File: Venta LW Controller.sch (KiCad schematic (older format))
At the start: 21 parts, among them J1 Conn_01x04, J2 Conn_02x05_Odd_Even, Q1 BSS138, Q2 BSS138, SW1 RST, SW2 FLASH, U1 LM2674N-3.3, U2 ESP32-WROOM-32

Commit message: updated parts
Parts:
- C1: footprint Capacitor_Tantalum_SMD:CP_EIA-3216-18_Kemet-A -> Capacitor_Tantalum_SMD:CP_EIA-7343-31_Kemet-D; Supplier Part TPSA226K010R0900 -> T491D226K035AT
- C4: Supplier Part CL03B103KP3NNNC -> CL21B103KBANNNC
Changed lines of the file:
@@
 F 0 "C1" H 1838 1696 50  0000 L CNN
 F 1 "22uF" H 1838 1605 50  0000 L CNN
-F 2 "Capacitor_Tantalum_SMD:CP_EIA-3216-18_Kemet-A" H 1750 1650 50  0001 C CNN
+F 2 "Capacitor_Tantalum_SMD:CP_EIA-7343-31_Kemet-D" H 1750 1650 50  0001 C CNN
 F 3 "~" H 1750 1650 50  0001 C CNN
 F 4 "TME" H 1750 1650 50  0001 C CNN "Supplier"
-F 5 "TPSA226K010R0900" H 1750 1650 50  0001 C CNN "Supplier Part"
+F 5 "T491D226K035AT" H 1750 1650 50  0001 C CNN "Supplier Part"
 	1    1750 1650
 	1    0    0    -1
@@
 F 3 "~" H 2600 2550 50  0001 C CNN
 F 4 "TME" H 2600 2550 50  0001 C CNN "Supplier"
-F 5 "CL03B103KP3NNNC" H 2600 2550 50  0001 C CNN "Supplier Part"
+F 5 "CL21B103KBANNNC" H 2600 2550 50  0001 C CNN "Supplier Part"
 	1    2600 2550
 	1    0    0    -1

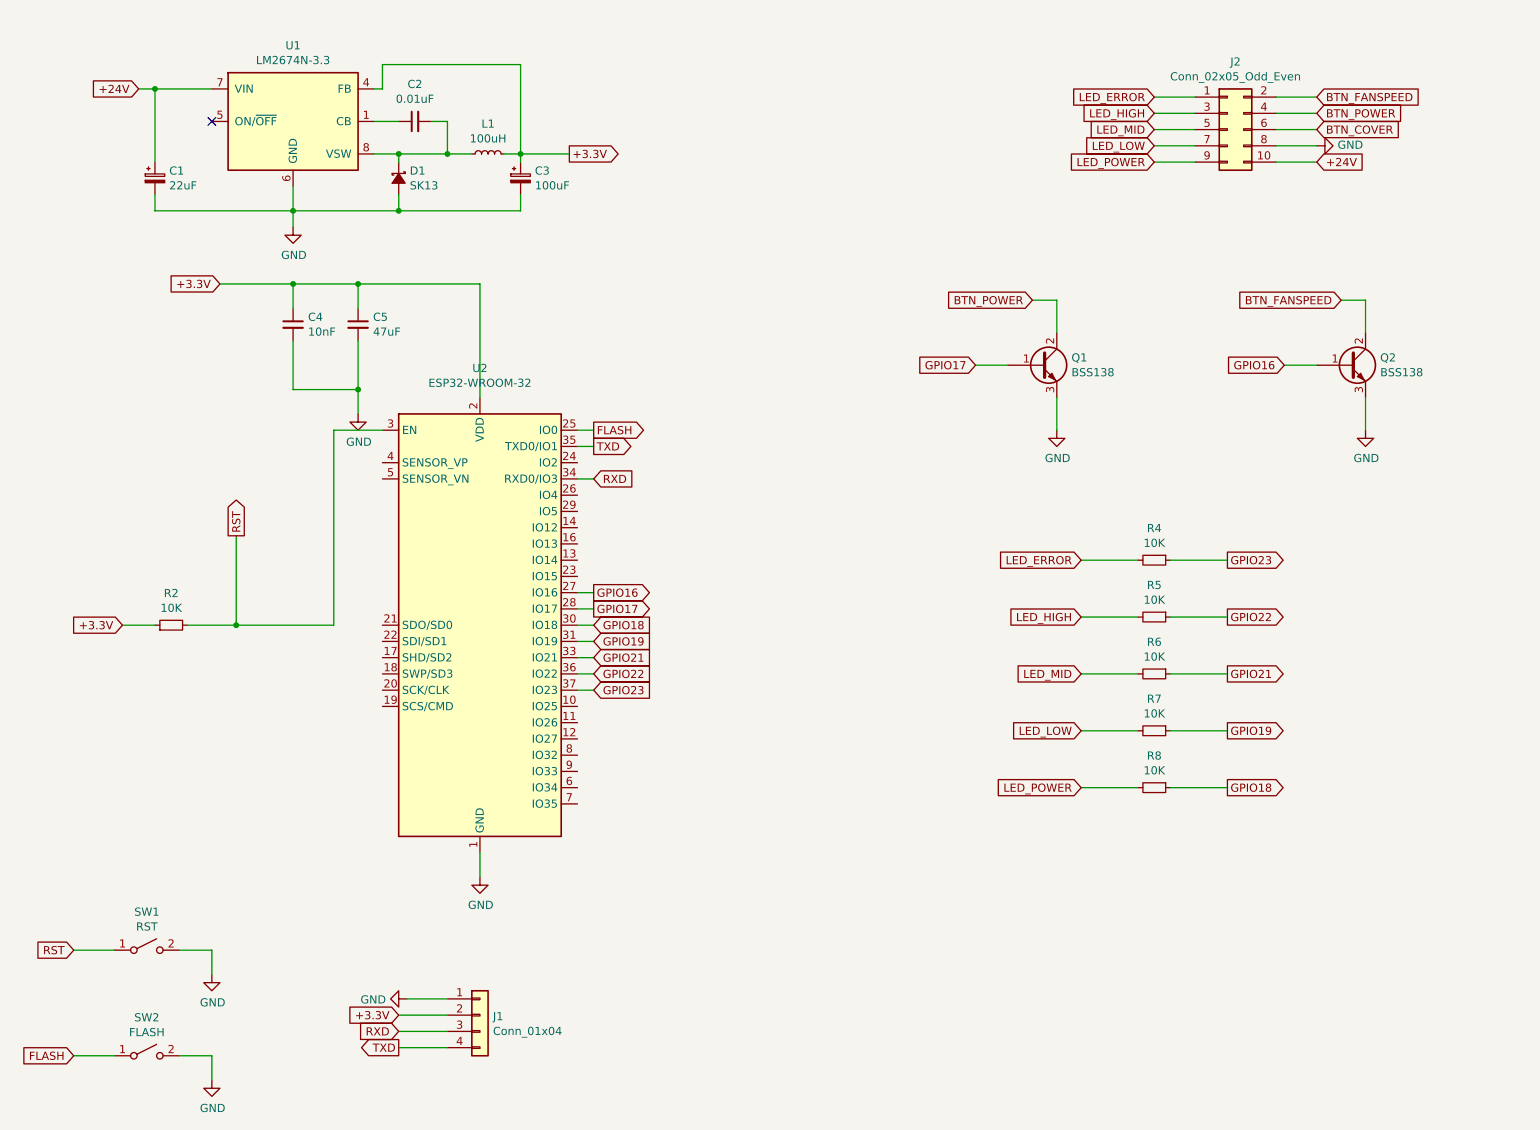
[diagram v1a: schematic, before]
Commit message: reworked
- added correct circuit for BSS138
- added voltage divider for inputs
- changed buck converter setup
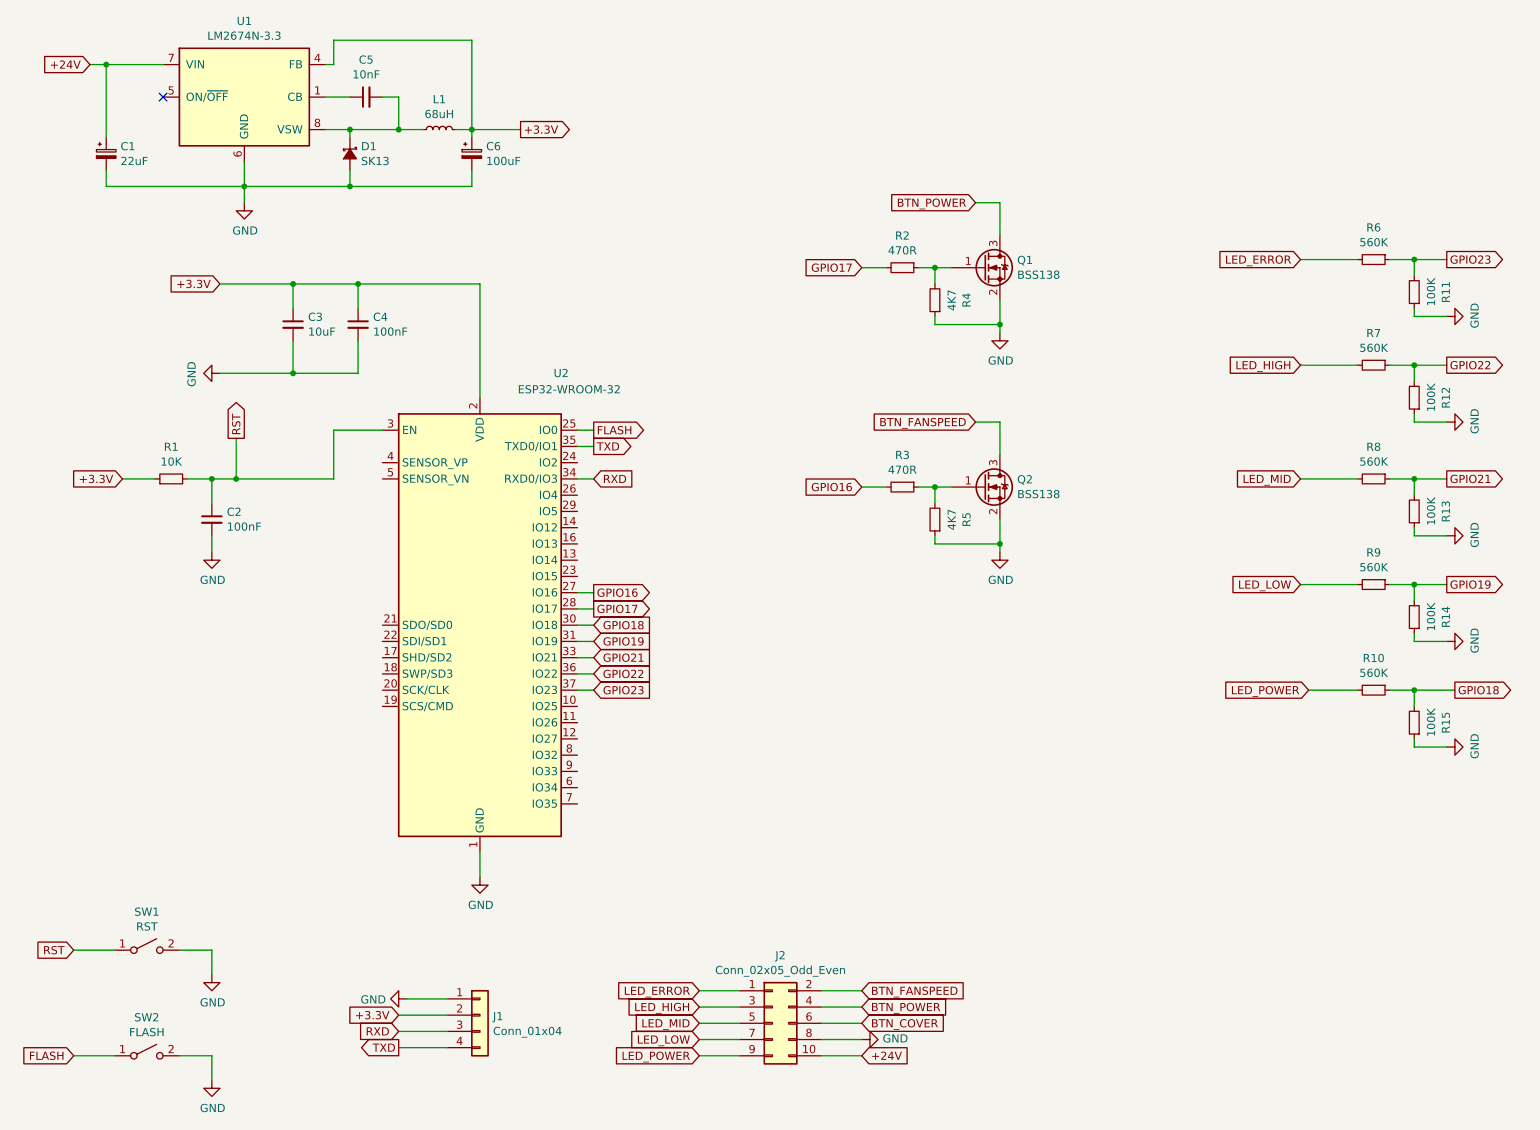
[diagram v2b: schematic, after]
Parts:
- removed Q1, Q2: BSS138, Package_TO_SOT_SMD:SOT-23, symbol Device:Q_NPN_BCE
- added C2: 100nF, Capacitor_SMD:C_0603_1608Metric, symbol Device:C_Small
- added Q1, Q2: BSS138, Package_TO_SOT_SMD:SOT-23, symbol Transistor_FET:BSS138
- added R11, R12, R13, R14, R15: 100K, Resistor_SMD:R_0603_1608Metric, symbol Device:R_Small
- added R2, R3: 470R, Resistor_SMD:R_0603_1608Metric, symbol Device:R_Small
- added R4, R5: 4K7, Resistor_SMD:R_0603_1608Metric, symbol Device:R_Small
- C1: Supplier Part T491D226K035AT -> TAJD226K035R
- C3: renamed from C4; value 10nF -> 10uF; footprint Capacitor_SMD:C_0805_2012Metric -> Capacitor_SMD:C_0603_1608Metric; Supplier Part CL21B103KBANNNC -> CL10A106KQ8NNNC
- C4: renamed from C5; value 47uF -> 100nF; footprint Capacitor_SMD:C_0805_2012Metric -> Capacitor_SMD:C_0603_1608Metric; Supplier TM -> TME; Supplier Part CL21A476MQYNNNG -> CL10B104KO8NNNC
- C5: renamed from C2; value 0.01uF -> 10nF; Supplier Part 06035A100JAT2A -> CL10B103KB8NNNC
- L1: value 100uH -> 68uH; footprint Inductor_SMD:L_12x12mm_H8mm -> Inductor_SMD:L_12x12mm_H6mm; Supplier Part DE1207-120 -> DE1205-68
- R10: renamed from R8; value 10K -> 560K; Supplier Part SMD0603-10K-1% -> SMD0603-560K-1%
- R6: renamed from R4; value 10K -> 560K; Supplier Part SMD0603-10K-1% -> SMD0603-560K-1%
- R7: renamed from R5; value 10K -> 560K; Supplier Part SMD0603-10K-1% -> SMD0603-560K-1%
- R8: renamed from R6; value 10K -> 560K; Supplier Part SMD0603-10K-1% -> SMD0603-560K-1%
- R9: renamed from R7; value 10K -> 560K; Supplier Part SMD0603-10K-1% -> SMD0603-560K-1%
- renumbered C3 to C6, R2 to R1
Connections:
- net BTN_FANSPEED: now also Q2.3 (D)
- net BTN_POWER: now also Q1.3 (D)
- net GND: now also C2.2, Q1.2 (S), Q2.2 (S), R11.1, R12.1, R13.1, R14.1, R15.1, R4.1, R5.1
- net GPIO16: now also R3.2
- net GPIO17: now also R2.2
- net GPIO18: now also R15.2
- net GPIO19: now also R14.2
- net GPIO21: now also R13.2
- net GPIO22: now also R12.2
- net GPIO23: now also R11.2
- net RST: now also C2.1
- new net: Q1.1 (G), R2.1, R4.2
- new net: Q2.1 (G), R3.1, R5.2
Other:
- moved on the sheet: C1, C5, C6, D1, J2, L1, R1, R10, R6, R7, R8, R9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
